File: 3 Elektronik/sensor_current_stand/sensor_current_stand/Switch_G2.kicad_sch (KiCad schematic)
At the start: 1 part, among them J6 DC37_Plug_MountingHoles

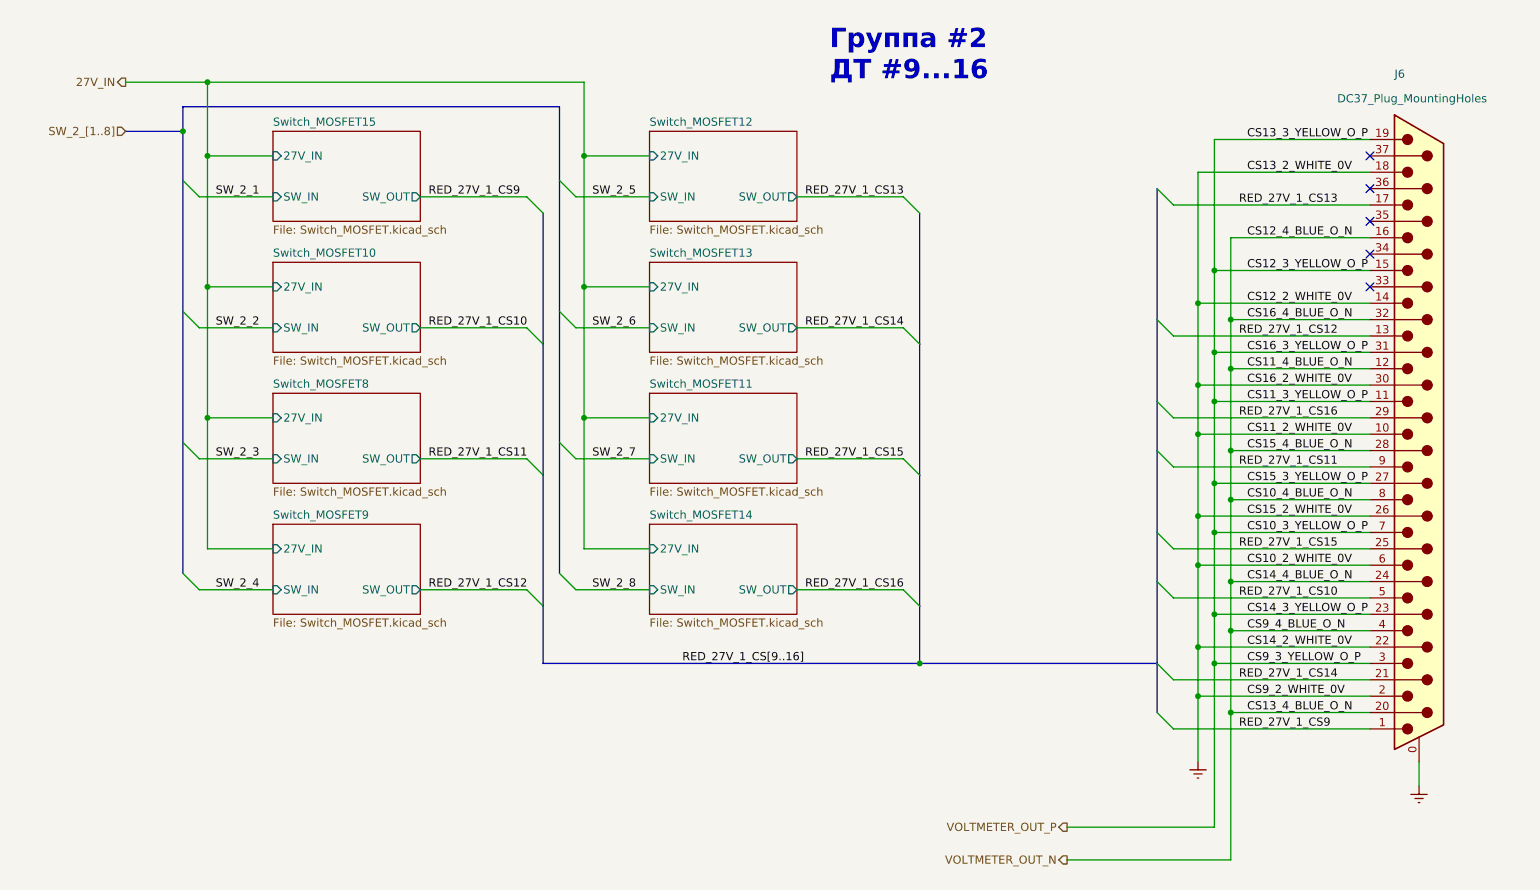
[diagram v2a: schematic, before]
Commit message: Version 2
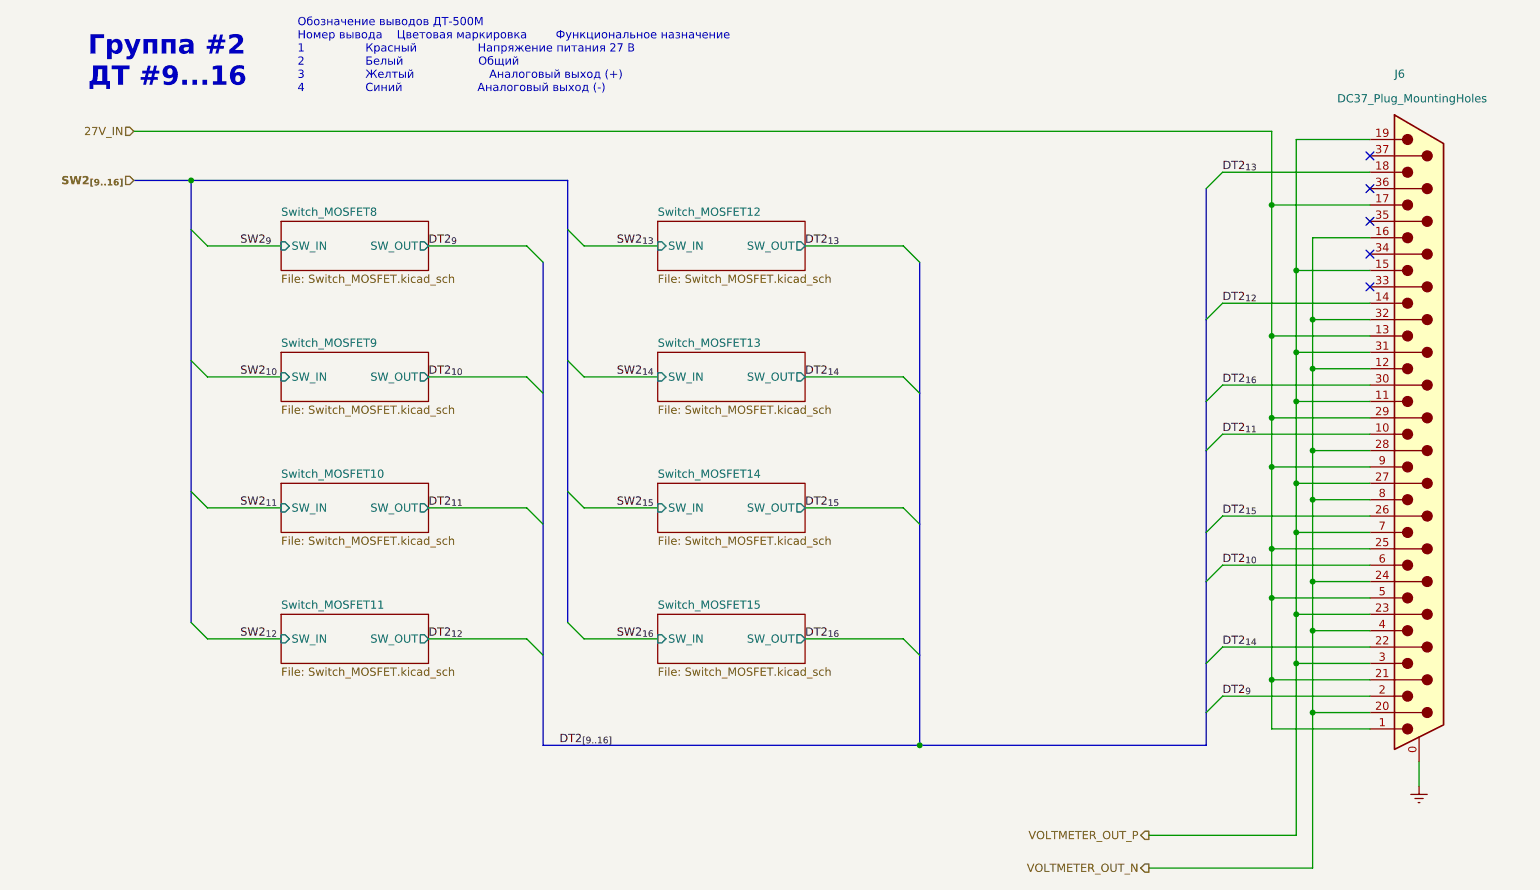
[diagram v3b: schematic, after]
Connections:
- net RED_27V_1_CS10 is gone; now on net 27V_IN: J6.5
- net RED_27V_1_CS11 is gone; now on net 27V_IN: J6.9
- net RED_27V_1_CS12 is gone; now on net 27V_IN: J6.13
- net RED_27V_1_CS13 is gone; now on net 27V_IN: J6.17
- net RED_27V_1_CS14 is gone; now on net 27V_IN: J6.21
- net RED_27V_1_CS15 is gone; now on net 27V_IN: J6.25
- net RED_27V_1_CS16 is gone; now on net 27V_IN: J6.29
- net RED_27V_1_CS9 is gone; now on net 27V_IN: J6.1
- net Earth: no longer J6.10, J6.14, J6.18, J6.2, J6.22, J6.26, J6.30, J6.6
- new net DT2_{10}: J6.6
- new net DT2_{11}: J6.10
- new net DT2_{12}: J6.14
- new net DT2_{13}: J6.18
- new net DT2_{14}: J6.22
- new net DT2_{15}: J6.26
- new net DT2_{16}: J6.30
- new net DT2_{9}: J6.2
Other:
- sheet Switch_MOSFET10 ports: added none; removed 27V_IN
- sheet Switch_MOSFET11 ports: added none; removed 27V_IN
- sheet Switch_MOSFET12 ports: added none; removed 27V_IN
- sheet Switch_MOSFET13 ports: added none; removed 27V_IN
- sheet Switch_MOSFET14 ports: added none; removed 27V_IN
- sheet Switch_MOSFET15 ports: added none; removed 27V_IN
- sheet Switch_MOSFET8 ports: added none; removed 27V_IN
- sheet Switch_MOSFET9 ports: added none; removed 27V_IN
- note added: "Обозначение выводов ДТ-500М Номер вывода Цветовая маркировка Функциональное назначение 1 Красный Напряжение питания 27 В 2 Белый Общий 3 Желтый Аналоговый выход (+) 4 Синий Аналоговый выход (-)"
